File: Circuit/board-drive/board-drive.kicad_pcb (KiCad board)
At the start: 2 copper layers, 164.3 x 98.3 mm, 33 parts, among them M3 MountingHole_3.2mm_M3, P1 XT30, P10 XT60, P2 XT30, P3 XT30, P4 XT30, P5 XT30, P6 XT30, P7 XT30, P8 XT30, P9 XT60, U1 Pololu_Maestro12, U10 PowerDist_WiretoBoard, U11 PowerDist_WiretoBoard, U16 PowerDist_WiretoBoard, U17 PowerDist_WiretoBoard, U18 PowerDist_WiretoBoard, U19 PowerDist_WiretoBoard, U2 Si8660BA-B-IS1, U3 Si8660BA-B-IS1, U8 PowerDist_WiretoBoard, U9 PowerDist_WiretoBoard

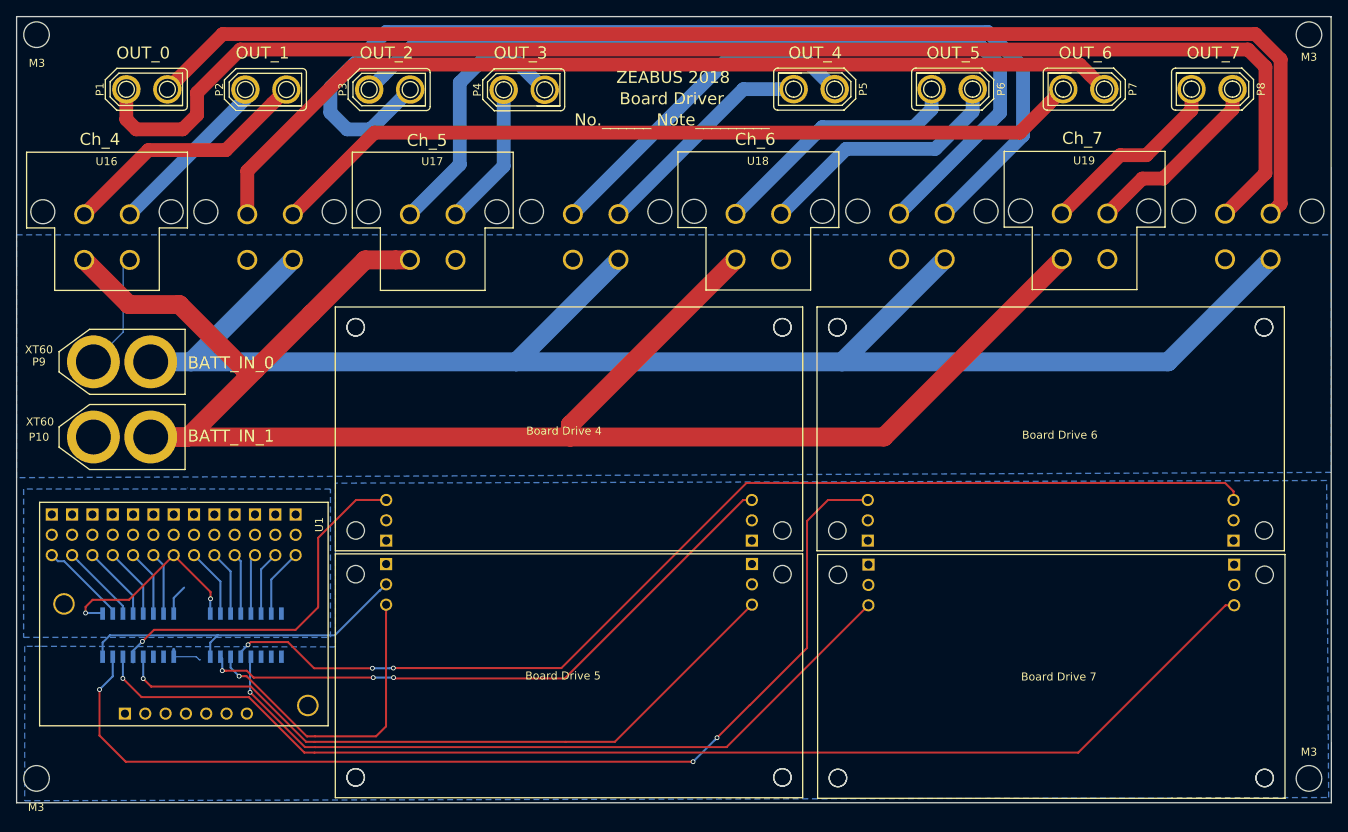
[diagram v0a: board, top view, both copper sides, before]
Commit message: edited pcb
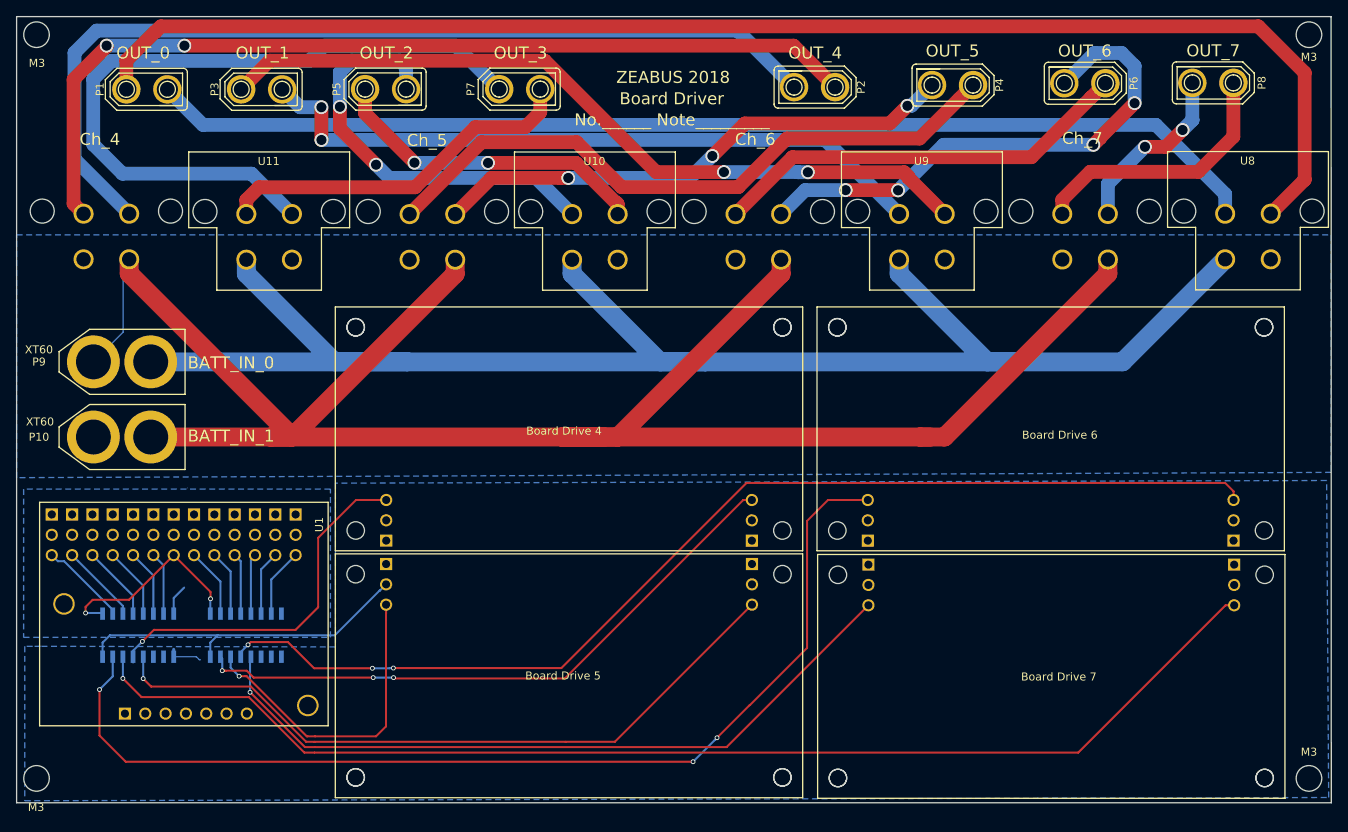
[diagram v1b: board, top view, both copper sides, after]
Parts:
- U10, U11, U8, U9: moved to F.Cu
- U16, U17, U18, U19: moved to B.Cu
- moved P7 70.1 mm to (113.2, 60.9), turned to 90 degrees
- moved P2 68.1 mm to (149.6, 60.7), turned to 270 degrees
- moved P5 53.1 mm to (96.4, 60.9), turned to 90 degrees
- moved P4 53.1 mm to (166.8, 60.4), turned to 270 degrees
- moved U11 25.0 mm to (69.2, 66.7), turned to 0 degrees
- moved U10 25.0 mm to (109.9, 66.7), turned to 0 degrees
- moved U19 25.0 mm to (196.0, 66.7), turned to 180 degrees
- moved U9 24.9 mm to (150.7, 66.7), turned to 0 degrees
- moved U18 24.9 mm to (155.2, 66.7), turned to 180 degrees
- moved U8 24.9 mm to (191.5, 66.6), turned to 0 degrees
- moved U17 24.9 mm to (114.5, 66.7), turned to 180 degrees
- moved U16 24.8 mm to (73.7, 66.6), turned to 180 degrees
- moved P6 16.6 mm to (183.3, 60.2)
- moved P3 16.0 mm to (80.9, 60.9)
- moved P8 0.79 mm to (199.3, 60.1)
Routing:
- net /OUTB_4: track 21.6 -> 116.4 mm, vias 0 -> 2
- net /OUTA_4: track 31.7 -> 117.0 mm
- net /OUTB_5: track 18.1 -> 81.8 mm
- net /OUTA_3: track 102.8 -> 45.9 mm
- net /OUTA_1: track 129.7 -> 86.0 mm, vias 0 -> 2
- net /OUTA_5: track 32.2 -> 66.3 mm, vias 0 -> 3
- net /OUTA_6: track 33.2 -> 65.7 mm, vias 0 -> 4
- net /OUTB_3: track 119.3 -> 91.3 mm
- net /OUTA_2: track 28.4 -> 52.7 mm, vias 0 -> 2
- net /OUTA_0: track 163.1 -> 140.1 mm
- net /OUTB_6: track 32.0 -> 53.0 mm
- net /BATTIN_1: track 222.5 -> 238.0 mm
- net /BATTIN_0: track 199.5 -> 210.4 mm
- net /OUTB_7: track 23.7 -> 33.2 mm
- net /OUTB_1: track 105.8 -> 97.4 mm, vias 0 -> 2
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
